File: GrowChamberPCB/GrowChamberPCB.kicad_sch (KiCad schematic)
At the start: 82 parts, among them J1 Screw_Terminal_01x02, J10 Screw_Terminal_01x03, J27 Conn_01x26_Pin, J3 TYPE-C-31-M-12, J7 Screw_Terminal_01x05, Q1 IRLML6244, Q2 IRLML6244, Q3 IRLML6244, Q4 IRLML6244, Q5 IRLML6244, Q6 IRLML6244, Q7 IRLR8721, Q9 IRLML6244, SW2 Reset, SW5 BootSwitch, U1 ESP32-S3-WROOM-1U, U2 MCP1826S, U3 USBLC6-2SC6, U4 TC4428xOA, U5 W25Q128JVS, U6 CR2013-MI2120

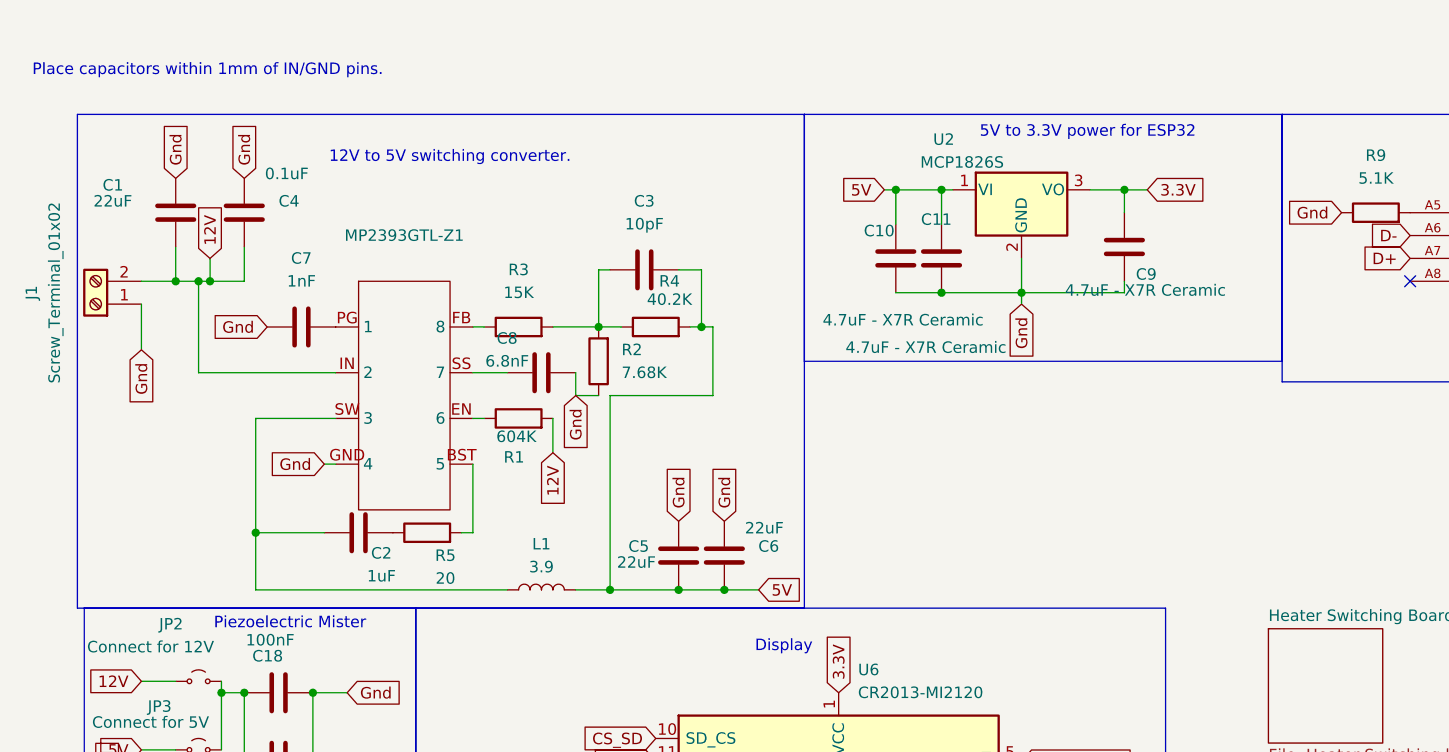
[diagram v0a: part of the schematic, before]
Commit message: added some BOM stuff
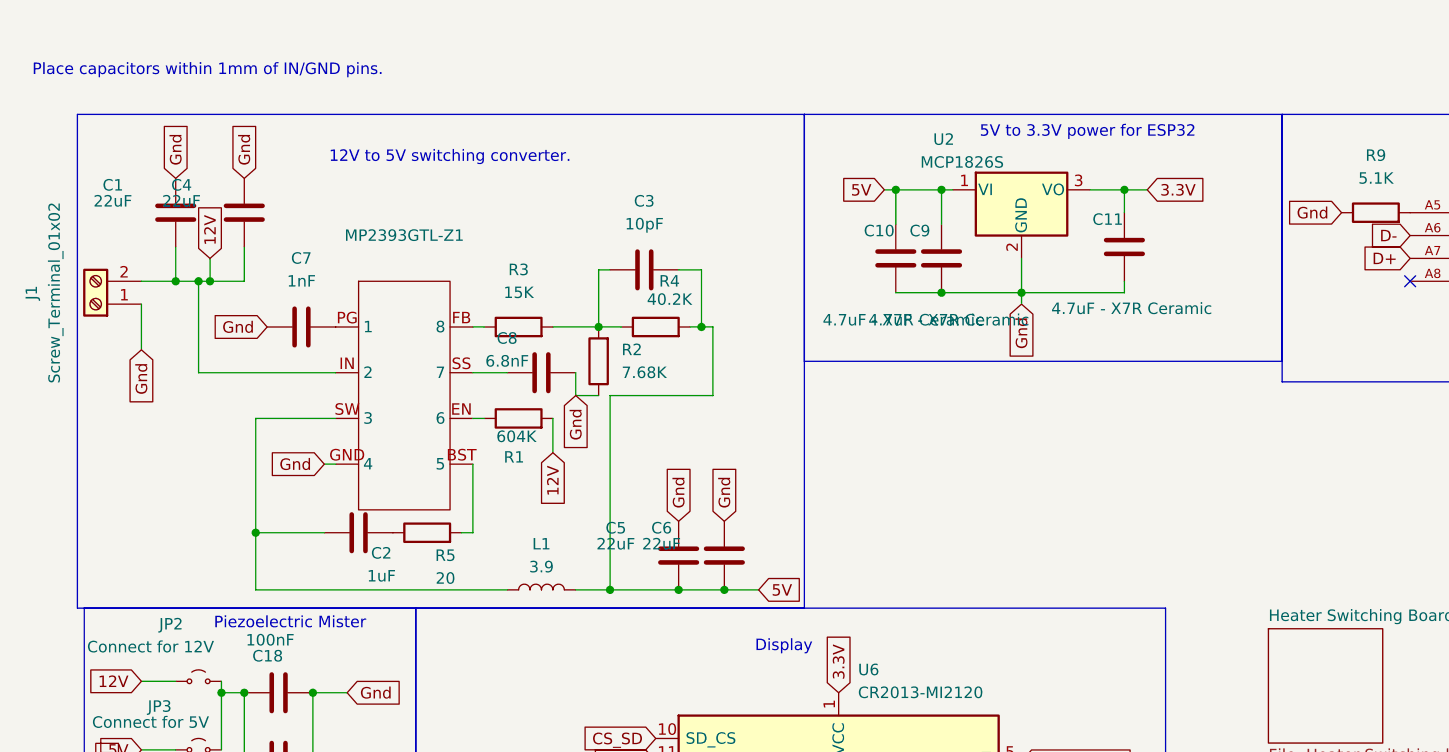
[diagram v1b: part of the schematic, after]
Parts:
- C1: footprint (none) -> digikey-footprints:0805; MFG Part Number GRM21BR61E226ME44L -> CL21A226KQCLRNC; Manufacturer (none) -> Samsung Electro-Mechanics; Package (none) -> 0805
- C10, C11, C9: footprint (none) -> digikey-footprints:0805; MFG Part Number (none) -> GRM21BR71C475KE51L; Manufacturer (none) -> Murata Electronics; Package (none) -> 0805 (2012 Metric); Type (SMD/thru-hole, etc.) (none) -> SMD
- C4: value 0.1uF -> 22uF; footprint (none) -> digikey-footprints:0805; MFG Part Number GRM188R71C105KA12D -> CL21A226KQCLRNC; Manufacturer (none) -> Samsung Electro-Mechanics; Package (none) -> 0805; Type (SMD/thru-hole, etc.) (none) -> SMD
- C5, C6: footprint (none) -> digikey-footprints:0805; MFG Part Number (none) -> CL21A226KQCLRNC; Manufacturer (none) -> Samsung Electro-Mechanics; Package (none) -> 0805; Type (SMD/thru-hole, etc.) (none) -> SMD
- J3: Availability Not in stock -> (none); Check_prices https://www.snapeda.com/parts/TYPE-C-31-M-12/HRO+Electronic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 -> (none); Description_1 USB Connectors 24 Receptacle 1 8.94*7.3mm RoHS -> (none); MANUFACTURER HRO Electronics Co., Ltd. -> (none); MAXIMUM_PACKAGE_HEIGHT 3.26 mm -> (none); MF HRO Electronics Co., Ltd. -> (none); MP TYPE-C-31-M-12 -> (none); PARTREV 2020.12.08 -> (none); Package/Footprint Package -> (none); Price None -> (none); SNAPEDA_PN TYPE-C-31-M-12 -> (none); STANDARD Manufacturer Recommendations -> (none); SnapEDA_Link https://www.snapeda.com/parts/TYPE-C-31-M-12/HRO+Electronic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 -> (none)
- U1: Availability Not in stock -> (none); Check_prices https://www.snapeda.com/parts/ESP32-S3-WROOM-1U/Espressif+S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 -> (none); Description_1 2.4 GHz Wi-Fi (802.11 b/g/n) and Bluetooth 5 (LE) module -> (none); MANUFACTURER Espressif -> (none); MAXIMUM_PACKAGE_HEIGHT 3.35mm -> (none); MF Espressif Systems -> (none); MP ESP32-S3-WROOM-1U -> (none); PARTREV v0.6 -> (none); Package/Footprint SMD-41 Espressif Systems -> (none); Price None -> (none); Purchase-URL https://www.snapeda.com/api/url_track_click_mouser/?unipart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 -> (none); STANDARD Manufacturer Recommendations -> (none); SnapEDA_Link https://www.snapeda.com/parts/ESP32-S3-WROOM-1U/Espressif+S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 -> (none)
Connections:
- net 3.3V: now also C11.1; no longer C9.1
- net 5V: now also C9.1; no longer C11.1

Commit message: BOM and footprints
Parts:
- C12, C13, C14, C15, C16, C17, C18, C19, C2, C20, C3, C7, C8, R1, R10, R11, R13, R14, R15, R16, R17, R18, R19, R2, R20, R21, R22, R23, R24, R25, R26, R27, R3, R30, R31, R32, R33, R4, R5, R6, R7, R8, R9: footprint (none) -> digikey-footprints:0805
- D2, D3, D4, D5, D6, D7, D8: footprint (none) -> Diode_SMD:D_SOD-123
- J1: footprint (none) -> TerminalBlock_RND:TerminalBlock_RND_205-00012_1x02_P5.00mm_Horizontal
- J10: footprint (none) -> Connector_Molex:Molex_KK-254_AE-6410-03A_1x03_P2.54mm_Vertical
- J27, SW2: footprint (none) -> Connector_PinHeader_2.54mm:PinHeader_2x13_P2.54mm_Vertical
- J7: footprint (none) -> Connector_Molex:Molex_KK-254_AE-6410-05A_1x05_P2.54mm_Vertical
- JP2, JP3: footprint (none) -> Jumper:SolderJumper-2_P1.3mm_Open_Pad1.0x1.5mm
- L1: footprint (none) -> Inductor_SMD:L_10.4x10.4_H4.8; MFG Part Number (none) -> SMDRH105R-3R3NT; Manufacturer (none) -> SXN(Shun Xiang Nuo Elec); Package (none) -> SMD, 10.4x10.3; Type (SMD/thru-hole, etc.) (none) -> SMD
- MP2393GTL-Z1: footprint (none) -> Package_TO_SOT_SMD:SOT-583-8
- Q1, Q2, Q3, Q4, Q5, Q6, Q7, Q9: footprint (none) -> digikey-footprints:SOT-23-3
- U5: footprint (none) -> digikey-footprints:SOIC-8_W5.3mm
- U6: footprint (none) -> Connector_PinHeader_2.54mm:PinHeader_1x14_P2.54mm_Vertical

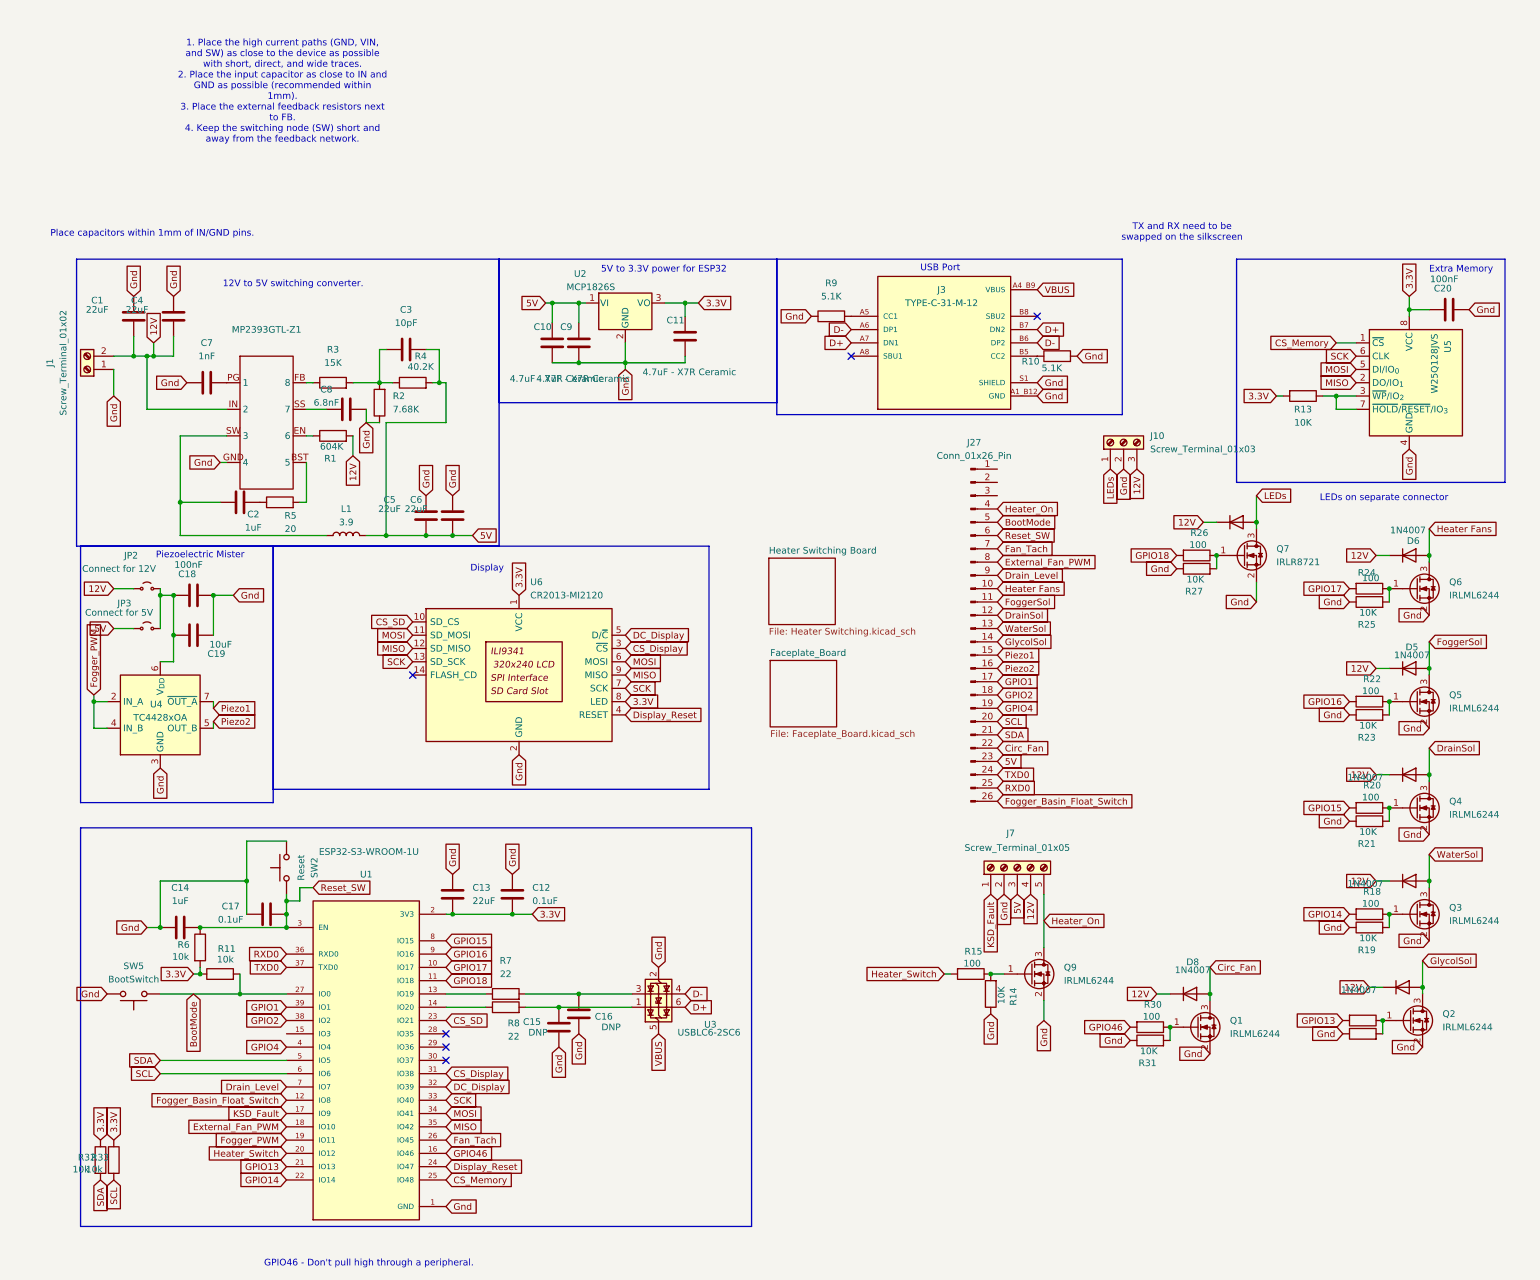
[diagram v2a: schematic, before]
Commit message: working on BOM and footprints
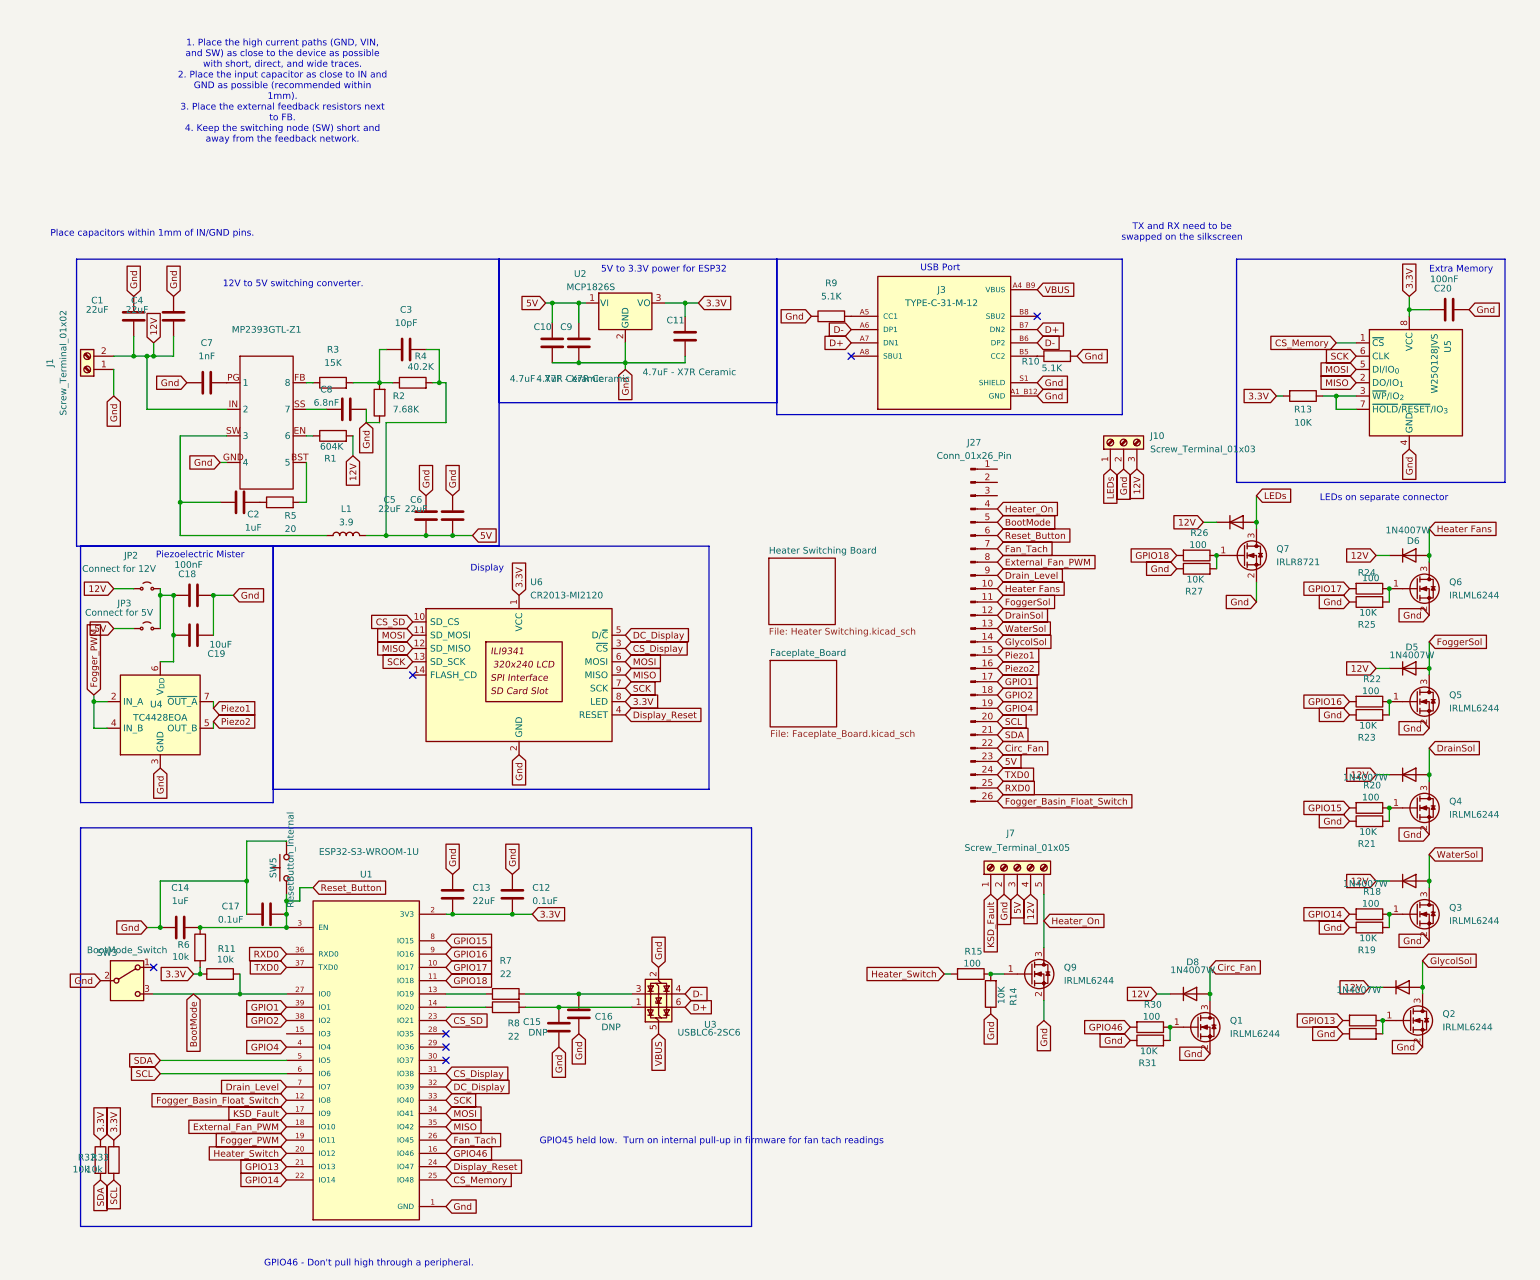
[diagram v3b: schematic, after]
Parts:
- removed SW2: Reset, Connector_PinHeader_2.54mm:PinHeader_2x13_P2.54mm_Vertical, symbol Switch:SW_Push
- added SW3: BootMode_Switch, symbol Switch:SW_SPDT
- D2, D3, D4, D5, D6, D7, D8: value 1N4007 -> 1N4007W; MFG Part Number (none) -> 1N4007W; Manufacturer (none) -> FUXINSEMI; Package (none) -> SMD
- J7: footprint Connector_Molex:Molex_KK-254_AE-6410-05A_1x05_P2.54mm_Vertical -> TerminalBlock_RND:TerminalBlock_RND_205-00015_1x05_P5.00mm_Horizontal
- SW5: value BootSwitch -> ResetButton_Internal; footprint (none) -> Button_Switch_SMD:SW_Push_1P1T_XKB_TS-1187A; MFG Part Number (none) -> TS-1187A-B-A-B; Manufacturer (none) -> XKB Connection; Package (none) -> SMD-4P,5.1x5.1mm; Type (SMD/thru-hole, etc.) (none) -> SMD
- U2: footprint (none) -> Package_TO_SOT_SMD:SOT-223-3_TabPin2; MFG Part Number (none) -> MCP1826S-3302E/DB; Manufacturer (none) -> Microchip Tech; Package (none) -> SOT-223-3; Type (SMD/thru-hole, etc.) (none) -> SMD
- U3: footprint (none) -> Package_TO_SOT_SMD:SOT-23-6_Handsoldering; MFG Part Number (none) -> USBLC6-2SC6; Manufacturer (none) -> STMicroelectronics; Package (none) -> SOT-23-6L; Type (SMD/thru-hole, etc.) (none) -> SMD
- U4: value TC4428xOA -> TC4428EOA; footprint (none) -> digikey-footprints:SOIC-8_W3.9mm; MFG Part Number (none) -> TC4428EOA; Manufacturer (none) -> Microchip Tech; Package (none) -> SOIC-8; Type (SMD/thru-hole, etc.) (none) -> SMD
- U5: footprint digikey-footprints:SOIC-8_W5.3mm -> Package_SO:SOIC-8_5.3x5.3mm_P1.27mm; MFG Part Number (none) -> W25Q128JVSIQ; Manufacturer (none) -> Winbond Ele; Package (none) -> SOIC-8 208-mil; Type (SMD/thru-hole, etc.) (none) -> SMD
- U6: MFG Part Number (none) -> NA; Manufacturer (none) -> NA; Package (none) -> pinholes; Type (SMD/thru-hole, etc.) (none) -> Through-hole
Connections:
- net BootMode: now also SW3.3 (C); no longer SW5.1
- net GND: now also SW3.2 (B)
- net Reset_SW renamed Reset_Button
- net Reset_Button: now also SW5.1
- no-connect marks 6 -> 7
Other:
- note added: "GPIO45 held low. Turn on internal pull-up in firmware for fan tach readings"
